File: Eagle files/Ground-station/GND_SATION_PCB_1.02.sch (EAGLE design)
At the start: 66 parts, among them IC1 BMP280, J1 USB4110GFA, J2 XT60-M, J3 B4B-XH-AM_(LF)(SN), J6 503182-1852, U1 AMS1117-5.0, U2 SOIC127P790X216-8NW25Q128JVJSQ, U3 AMS1117-3.3

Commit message: .
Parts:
- added C21, C25, C26: 10uF, rcl:C-EUC0603
- added C27, C28, C29: (no value), rcl:C-EUC0603
- added D3, D4: SS14, SS14:SS14
- added J4: USB4110GFA, USB4110GFA:USB4110GFA
- added J5: XT60-M, XT60-M:XT60-M
- added R22, R23: 5.1 K, standardparts:RESISTOR.0603
- added R24: 10k ohm, standardparts:RESISTOR.0603
- added U4: SOIC127P790X216-8NW25Q128JVJSQ, SOIC127P790X216-8N:SOIC127P790X216-8NW25Q128JVJSQ
- added U5: AMS1117-3.3, AMS1117-3.3:AMS1117-3.3
- added U6: AMS1117-5.0, AMS1117-5.0:AMS1117-5.0
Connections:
- new net FLASH_CLK: U4.CLK
- new net FLASH_CS: R24.1, U4./CS
- new net FLASH_DI: U4.DI(IO0)
- new net FLASH_DO: U4.DO(I01)
- new net N$13: J4.CC1, R22.2
- new net N$20: J4.CC2, R23.2
- new net N$21: D3.A, J4.VBUS
- new net N$22: C27.2, C28.2, C29.2, U6.GND/ADJ
- new net N$23: C27.1, J5.NEG, U6.VIN
- new net N$24: C21.1, D3.K, D4.K, U5.VIN
- net 3V3: now also C25.1, C26.1, R24.2, U4./HOLD(IO3), U4./WP(IO2), U4.VCC, U5.VOUT
- net 5V_OUT: now also C28.1, C29.1, D4.A, U6.VOUT
- net D_N: now also J4.DN1, J4.DN2
- net D_P: now also J4.DP1, J4.DP2
- net GND: now also C21.2, C25.2, C26.2, J4.GND, J5.POS, R22.1, R23.1, U4.GND, U5.GND/ADJ
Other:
- note added: "Mismatch in footprint and actual chip"
- note added: "REDO"
- moved on the sheet: C1, C10, C11, C115, C12, C13, C14, C15, C16, C17, C18, C19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

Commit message: revision 1
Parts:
- removed C23, C24, C25, C26: 10uF, rcl:C-EUC0603
- removed C27, C28, C29: (no value), rcl:C-EUC0603
- removed D2, D3, D4: SS14, SS14:SS14
- removed J4: USB4110GFA, USB4110GFA:USB4110GFA
- removed J5: XT60-M, XT60-M:XT60-M
- removed R15, R23: 5.1 K, standardparts:RESISTOR.0603
- removed R19: 10k ohm, standardparts:RESISTOR.0603
- removed S1: DTS-3, DTS-3:DTS-3
- removed U2: SOIC127P790X216-8NW25Q128JVJSQ, SOIC127P790X216-8N:SOIC127P790X216-8NW25Q128JVJSQ
- removed U5: AMS1117-3.3, AMS1117-3.3:AMS1117-3.3
- removed U6: AMS1117-5.0, AMS1117-5.0:AMS1117-5.0
- added S3: DTS-3, DTS-3:DTS-3
- added U$3: ASE, crystal:ASE
- C1, C2: device ngspice-simulation:C -> rcl:C-EUC0805
- C13, C14, C21, C22: device rcl:C-EUC0603 -> rcl:C-EUC0805
- C17, C18, C19: value (none) -> 10uF; device rcl:C-EUC0603 -> rcl:C-EUC0805
- C3: value 100nF -> 10uF; device rcl:C-EUC0603 -> rcl:C-EUC0805
- R10: value 5.1 K -> 5.1k; device standardparts:RESISTOR.0603 -> rcl:R-EU_R0805
- R22: value 5.1 K -> 10k; device standardparts:RESISTOR.0603 -> rcl:R-EU_R0805
- R6: value 10k ohm -> 10k; device standardparts:RESISTOR.0603 -> rcl:R-EU_R0805
- R7: value 10k ohm -> 5.1k; device standardparts:RESISTOR.0603 -> rcl:R-EU_R0805
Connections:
- removed net N$11: J1.CC1, R10.2
- removed net N$13: J4.CC1, R22.2
- removed net N$17: C22.1, D1.K, D2.K, U3.VIN
- removed net N$20: J4.CC2, R23.2
- removed net N$21: D3.A, J4.VBUS
- removed net N$22: C27.2, C28.2, C29.2, U6.GND/ADJ
- removed net N$23: C27.1, J5.NEG, U6.VIN
- removed net N$24: C21.1, D3.K, D4.K, U5.VIN
- net +3V3: no longer C3.1, R7.2, U2.VCC
- net 3V3: now also C1.2, C19.1, C21.1; no longer C1.1, C23.1, C24.1, C25.1, C26.1, U5.VOUT
- net 5V_OUT: now also C17.1, C22.1, C3.1, U3.VIN; no longer C18.1, C19.1, C28.1, C29.1, D2.A, D4.A, U6.VOUT
- net D_N: no longer J4.DN1, J4.DN2
- net D_P: no longer J4.DP1, J4.DP2
- net FLASH_CS: now also R22.2
- net GND: now also C1.1, C17.2, C18.2, C19.2, J2.NEG, R7.1, S3.1, U1.GND/ADJ; no longer C1.2, C23.2, C24.2, C25.2, C26.2, J2.POS, J4.GND, J5.POS, R15.1, R22.1, R23.1, S1.1, U2.GND, U5.GND/ADJ
- net N$15: now also R10.2; no longer R15.2
- net N$16: now also C18.1, J2.POS; no longer C17.1, J2.NEG
- net N$2: now also R22.1, S3.2; no longer C17.2, C18.2, C19.2, U1.GND/ADJ
- net N$4: now also C14.2; no longer C13.2
- net N$5: now also J1.CC1, R7.2; no longer R19.1, S1.2
- net QSPI_SCLK: no longer U2.CLK
- net QSPI_SD0: no longer U2.DI(IO0)
- net QSPI_SD1: no longer U2.DO(I01)
- net QSPI_SD2: no longer U2./WP(IO2)
- net QSPI_SD3: no longer U2./HOLD(IO3)
- net QSPI_SS: no longer R19.2, R7.1, U2./CS
- net XIN: now also C13.2; no longer C14.2
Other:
- note added: "Crystal Oscillator"
- note added: "Flash chip (W25Q125JV)"
- note added: "Power Supply"
- moved on the sheet: C1, C13, C14, C17, C18, C19, C2, C21, C3, IC1, J2, R24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

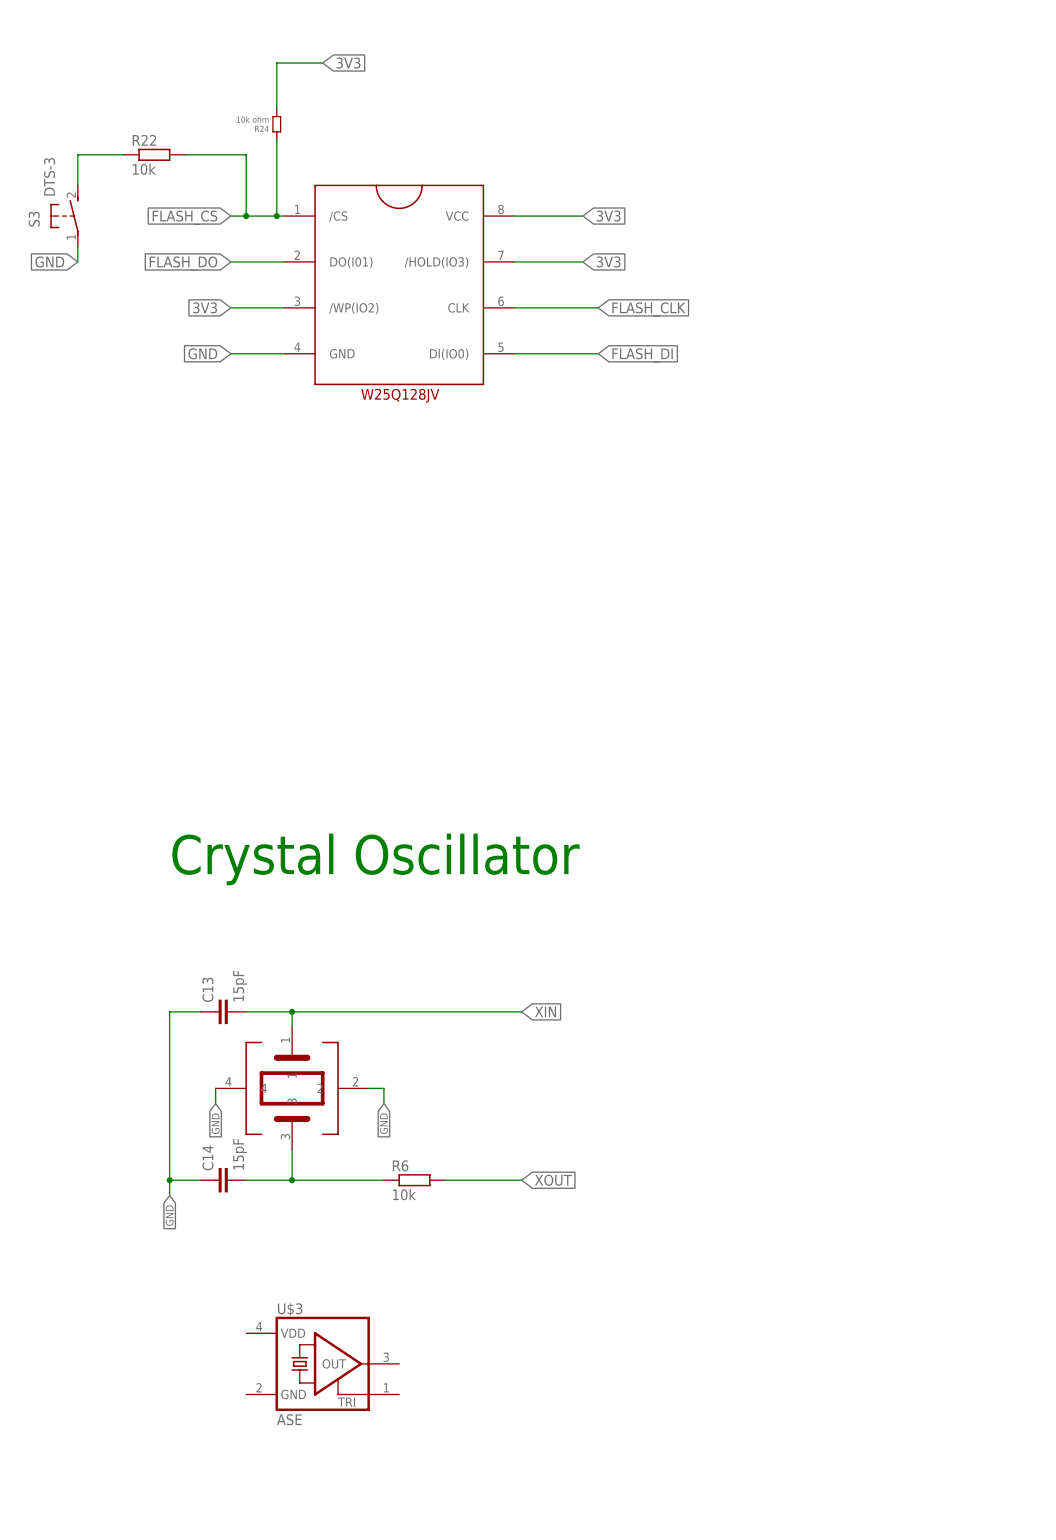
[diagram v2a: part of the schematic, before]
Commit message: Revision 1.01
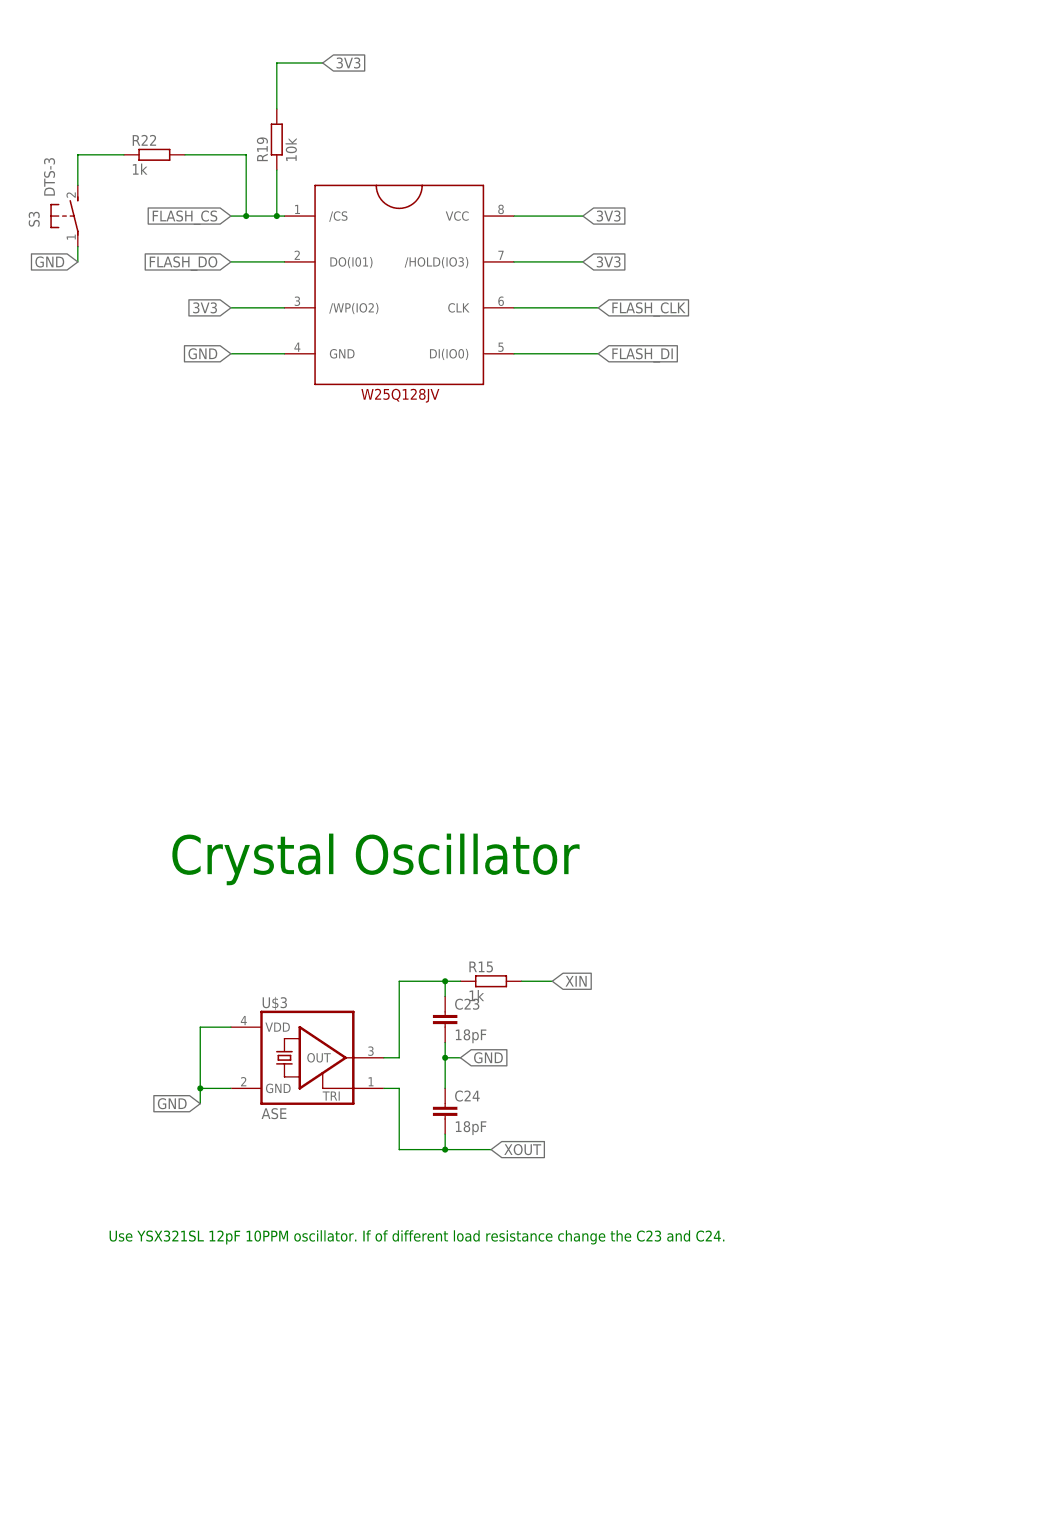
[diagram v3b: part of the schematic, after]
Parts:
- removed C13, C14: 15pF, rcl:C-EUC0805
- removed R24: 10k ohm, standardparts:RESISTOR.0603
- removed R6: 10k, rcl:R-EU_R0805
- removed U$1: ABM8-272-T3, ABM8-272-T3:ABM8-272-T3
- added C23, C24: 18pF, rcl:C-EUC0805
- added R15: 1k, rcl:R-EU_R0805
- added R19: 10k, rcl:R-EU_R0805
- R22: value 10k -> 1k
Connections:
- removed net N$4: C14.2, R6.1, U$1.3
- new net N$11: C23.1, R15.1, U$3.OUT
- net 3V3: now also R19.2; no longer R24.2
- net FLASH_CS: now also R19.1; no longer R24.1
- net GND: now also C23.2, C24.1, U$3.GND, U$3.VDD; no longer C13.1, C14.1, U$1.2, U$1.4
- net XIN: now also R15.2; no longer C13.2, U$1.1
- net XOUT: now also C24.2, U$3.TRI; no longer R6.2
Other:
- note added: "Use YSX321SL 12pF 10PPM oscillator. If of different load resistance change the C23 and C24."
- moved on the sheet: U$3
